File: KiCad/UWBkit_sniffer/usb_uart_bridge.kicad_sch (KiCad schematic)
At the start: 9 parts, among them U2 CP2104

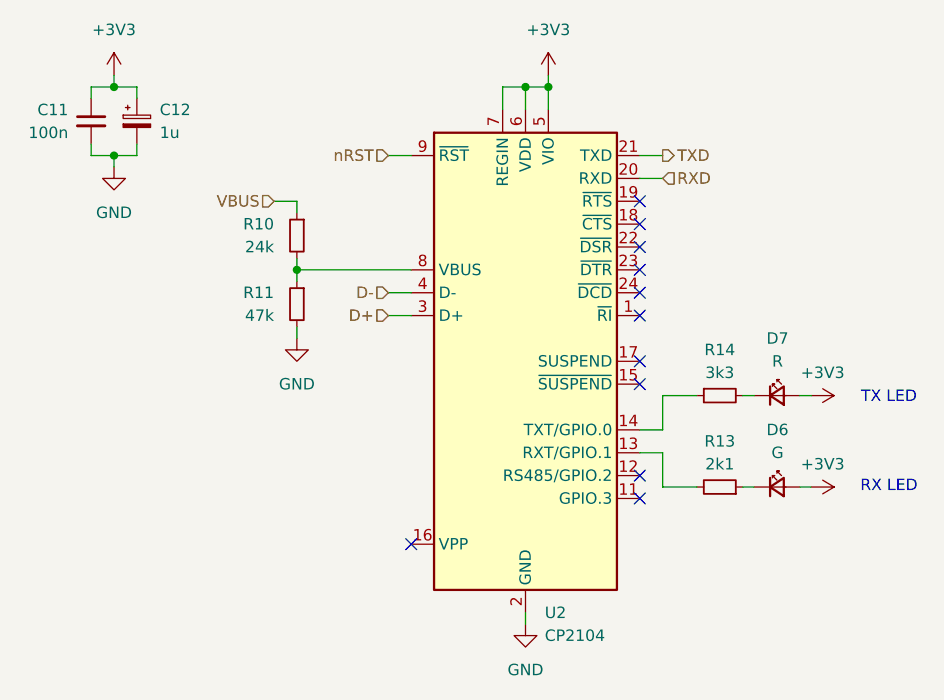
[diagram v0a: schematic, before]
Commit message: First version of PCB
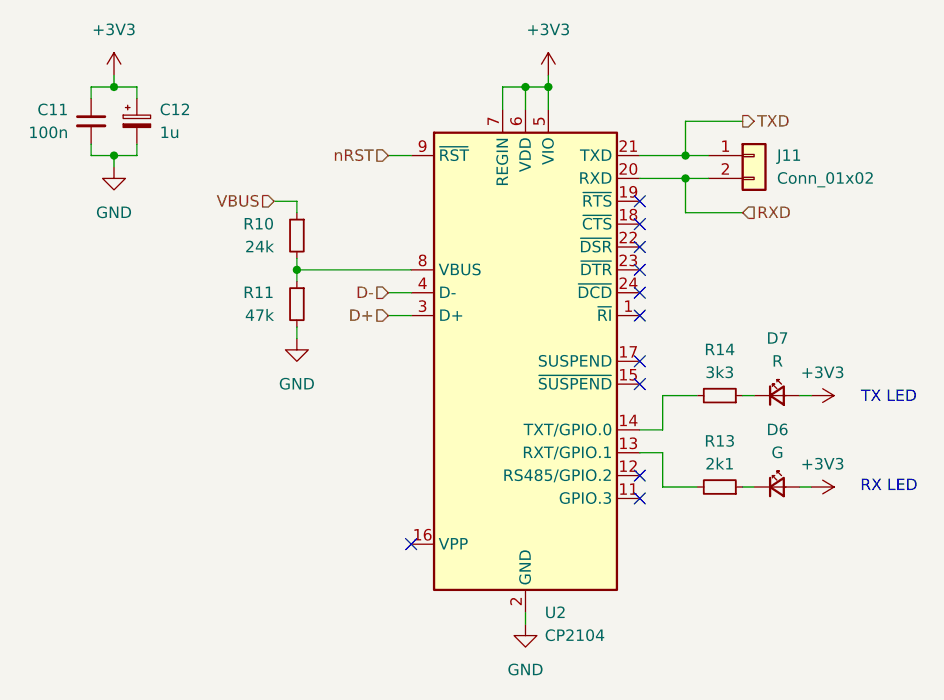
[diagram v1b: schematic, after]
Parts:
- added J11: Conn_01x02, Connector_PinHeader_2.54mm:PinHeader_1x02_P2.54mm_Vertical, symbol Connector_Generic:Conn_01x02
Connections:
- net RXD: now also J11.2 (Pin_2)
- net TXD: now also J11.1 (Pin_1)
- net at U2.14 (TXT/GPIO.0): now also R14.2; no longer R14.1
- net at D7.1 (K): now also R14.1; no longer R14.2
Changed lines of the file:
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@@
+	)
+	(junction
+		(at 166.37 72.39)
+		(diameter 0)
+		(color 0 0 0 0)
 	)
 	(junction
@@
 		(color 0 0 0 0)
 	)
+	(junction
+		(at 166.37 69.85)
+		(diameter 0)
+		(color 0 0 0 0)
+	)
 	(no_connect
 		(at 161.29 80.01)
@@
 	(wire
 		(pts
+			(xy 172.72 76.2) (xy 166.37 76.2)
+		)
+		(stroke
+			(width 0)
+			(type default)
+		)
+	)
+	(wire
+		(pts
+			(xy 166.37 72.39) (xy 168.91 72.39)
+		)
+		(stroke
+			(width 0)
+			(type default)
+		)
+	)
+	(wire
+		(pts
 			(xy 146.05 62.23) (xy 148.59 62.23)
 		)
@@
 	(wire
 		(pts
+			(xy 172.72 66.04) (xy 166.37 66.04)
+		)
+		(stroke
+			(width 0)
+			(type default)
+		)
+	)
+	(wire
+		(pts
 			(xy 102.87 69.85) (xy 102.87 71.12)
 		)
@@
 	(wire
 		(pts
-			(xy 161.29 69.85) (xy 163.83 69.85)
+			(xy 161.29 69.85) (xy 166.37 69.85)
 		)
 		(stroke
@@
 	(wire
 		(pts
+			(xy 166.37 69.85) (xy 168.91 69.85)
+		)
+		(stroke
+			(width 0)
+			(type default)
+		)
+	)
+	(wire
+		(pts
 			(xy 105.41 68.58) (xy 105.41 69.85)
 		)
@@
 	(wire
 		(pts
+			(xy 166.37 76.2) (xy 166.37 72.39)
+		)
+		(stroke
+			(width 0)
+			(type default)
+		)
+	)
+	(wire
+		(pts
 			(xy 173.99 106.68) (xy 172.72 106.68)
 		)
@@
 	(wire
 		(pts
-			(xy 161.29 72.39) (xy 163.83 72.39)
+			(xy 166.37 66.04) (xy 166.37 69.85)
+		)
+		(stroke
+			(width 0)
+			(type default)
+		)
+	)
+	(wire
+		(pts
+			(xy 161.29 72.39) (xy 166.37 72.39)
 		)
 		(stroke
@@
 		)
 	)
+	(hierarchical_label "RXD"
+		(shape input)
+		(at 172.72 76.2 0)
+		(effects
+			(font
+				(size 1.27 1.27)
+			)
+			(justify left)
+		)
+	)
 	(hierarchical_label "VBUS"
 		(shape input)
@@
 		)
 	)
-	(hierarchical_label "RXD"
-		(shape input)
-		(at 163.83 72.39 0)
-		(effects
-			(font
-				(size 1.27 1.27)
-			)
-			(justify left)
-		)
-	)
 	(hierarchical_label "nRST"
 		(shape input)
@@
 	(hierarchical_label "TXD"
 		(shape output)
-		(at 163.83 69.85 0)
+		(at 172.72 66.04 0)
 		(effects
 			(font
@@
 	)
 	(symbol
-		(lib_id "Device:R_Small")
-		(at 170.18 96.52 90)
-		(mirror x)
-		(unit 1)
-		(exclude_from_sim no)
-		(in_bom yes)
-		(on_board yes)
-		(dnp no)
-		(fields_autoplaced yes)
-		(property "Reference" "R14"
-			(at 170.18 91.44 90)
-			(effects
-				(font
-					(size 1.27 1.27)
-				)
-			)
-		)
-		(property "Value" "3k3"
-			(at 170.18 93.98 90)
-			(effects
-				(font
-					(size 1.27 1.27)
-				)
-			)
-		)
-		(property "Footprint" "Resistor_SMD:R_0603_1608Metric"
-			(at 170.18 96.52 0)
-			(effects
-				(font
-					(size 1.27 1.27)
-				)
-				(hide yes)
-			)
-		)
-		(property "Datasheet" "~"
-			(at 170.18 96.52 0)
-			(effects
-				(font
-					(size 1.27 1.27)
-				)
-				(hide yes)
-			)
-		)
-		(property "Description" "Resistor, small symbol"
-			(at 170.18 96.52 0)
-			(effects
-				(font
-					(size 1.27 1.27)
-				)
-				(hide yes)
-			)
-		)
-		(pin "1"
-		)
-		(pin "2"
-		)
-		(instances
-			(project "UWBkit_sniffer"
-				(path "/7666dc1a-7b28-48ea-a5e3-eea89f700cea/69acd281-5c2d-45c7-b47b-523f2587d598"
-					(reference "R14")
-					(unit 1)
-				)
-			)
-		)
-	)
-	(symbol
 		(lib_id "Device:LED_Small")
 		(at 176.53 106.68 0)
@@
 					(unit 1)
 				)
+			)
+		)
+	)
+	(symbol
+		(lib_id "Connector_Generic:Conn_01x02")
+		(at 173.99 69.85 0)
+		(unit 1)
+		(exclude_from_sim no)
+		(in_bom yes)
+		(on_board yes)
+		(dnp no)
+		(fields_autoplaced yes)
+		(property "Reference" "J11"
+			(at 176.53 69.8499 0)
+			(effects
+				(font
+					(size 1.27 1.27)
+				)
+				(justify left)
+			)
+		)
+		(property "Value" "Conn_01x02"
+			(at 176.53 72.3899 0)
+			(effects
+				(font
+					(size 1.27 1.27)
+				)
+				(justify left)
+			)
+		)
+		(property "Footprint" "Connector_PinHeader_2.54mm:PinHeader_1x02_P2.54mm_Vertical"
+			(at 173.99 69.85 0)
+			(effects
+				(font
+					(size 1.27 1.27)
+				)
+				(hide yes)
+			)
+		)
+		(property "Datasheet" "~"
+			(at 173.99 69.85 0)
+			(effects
+				(font
+					(size 1.27 1.27)
+				)
+				(hide yes)
+			)
+		)
+		(property "Description" "Generic connector, single row, 01x02, script generated (kicad-library-utils/schlib/autogen/connector/)"
+			(at 173.99 69.85 0)
+			(effects
+				(font
+					(size 1.27 1.27)
+				)
+				(hide yes)
+			)
+		)
+		(pin "2"
+		)
+		(pin "1"
+		)
+		(instances
+			(project ""
+				(path "/7666dc1a-7b28-48ea-a5e3-eea89f700cea/69acd281-5c2d-45c7-b47b-523f2587d598"
+					(reference "J11")
+					(unit 1)
+				)
+			)
+		)
+	)
+	(symbol
+		(lib_id "Device:R_Small")
+		(at 170.18 96.52 270)
+		(mirror x)
+		(unit 1)
+		(exclude_from_sim no)
+		(in_bom yes)
+		(on_board yes)
+		(dnp no)
+		(fields_autoplaced yes)
+		(property "Reference" "R14"
+			(at 170.18 91.44 90)
+			(effects
+				(font
+					(size 1.27 1.27)
+				)
+			)
+		)
+		(property "Value" "3k3"
+			(at 170.18 93.98 90)
+			(effects
+				(font
+					(size 1.27 1.27)
+				)
+			)
+		)
+		(property "Footprint" "Resistor_SMD:R_0603_1608Metric"
+			(at 170.18 96.52 0)
+			(effects
+				(font
+					(size 1.27 1.27)
+				)
+				(hide yes)
+			)
+		)
+		(property "Datasheet" "~"
+			(at 170.18 96.52 0)
+			(effects
+				(font
+					(size 1.27 1.27)
+				)
+				(hide yes)
+			)
+		)
+		(property "Description" "Resistor, small symbol"
+			(at 170.18 96.52 0)
+			(effects
+				(font
+					(size 1.27 1.27)
+				)
+				(hide yes)
+			)
+		)
+		(pin "1"
+		)
+		(pin "2"
+		)
+		(instances
+			(project "UWBkit_sniffer"
+				(path "/7666dc1a-7b28-48ea-a5e3-eea89f700cea/69acd281-5c2d-45c7-b47b-523f2587d598"
+					(reference "R14")
+					(unit 1)
+				)
